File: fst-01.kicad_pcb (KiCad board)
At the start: 2 copper layers, 21.2 x 12.6 mm, 17 parts, among them J1 USB_A, K1 CONN_3, U1 STM32F103TB, U2 MCP1700-3302E, U3 NUF2221W1, U4 X2SON, X1 12MHz

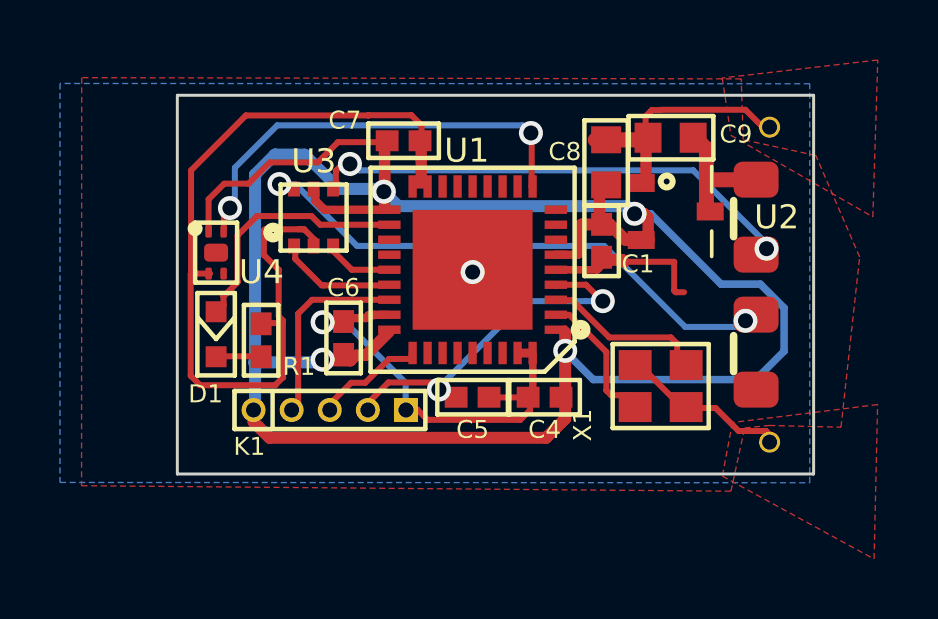
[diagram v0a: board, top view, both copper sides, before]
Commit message: Ask PCBA quote with this.
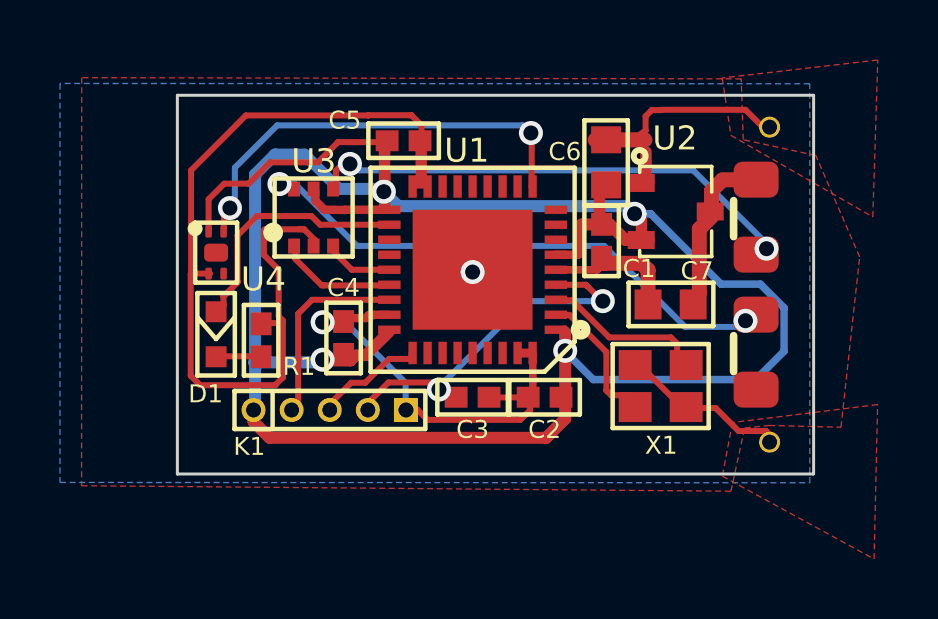
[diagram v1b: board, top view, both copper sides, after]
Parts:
- moved C7 5.56 mm to (124.9, 99.7)
- renumbered C4 to C2, C5 to C3, C6 to C4, C7 to C5, C8 to C6, C9 to C7
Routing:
- net GND: track 75.4 -> 74.1 mm
- net /VBUS: track 3.93 -> 4.65 mm
